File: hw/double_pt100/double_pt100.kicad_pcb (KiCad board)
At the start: 2 copper layers, 88.9 x 45.7 mm, 30 parts, among them SW1 SW_Push, U1 WeMos_D1_mini, U2 OLED_091_module, U3 MAX31865_breakout, U4 MAX31865_breakout

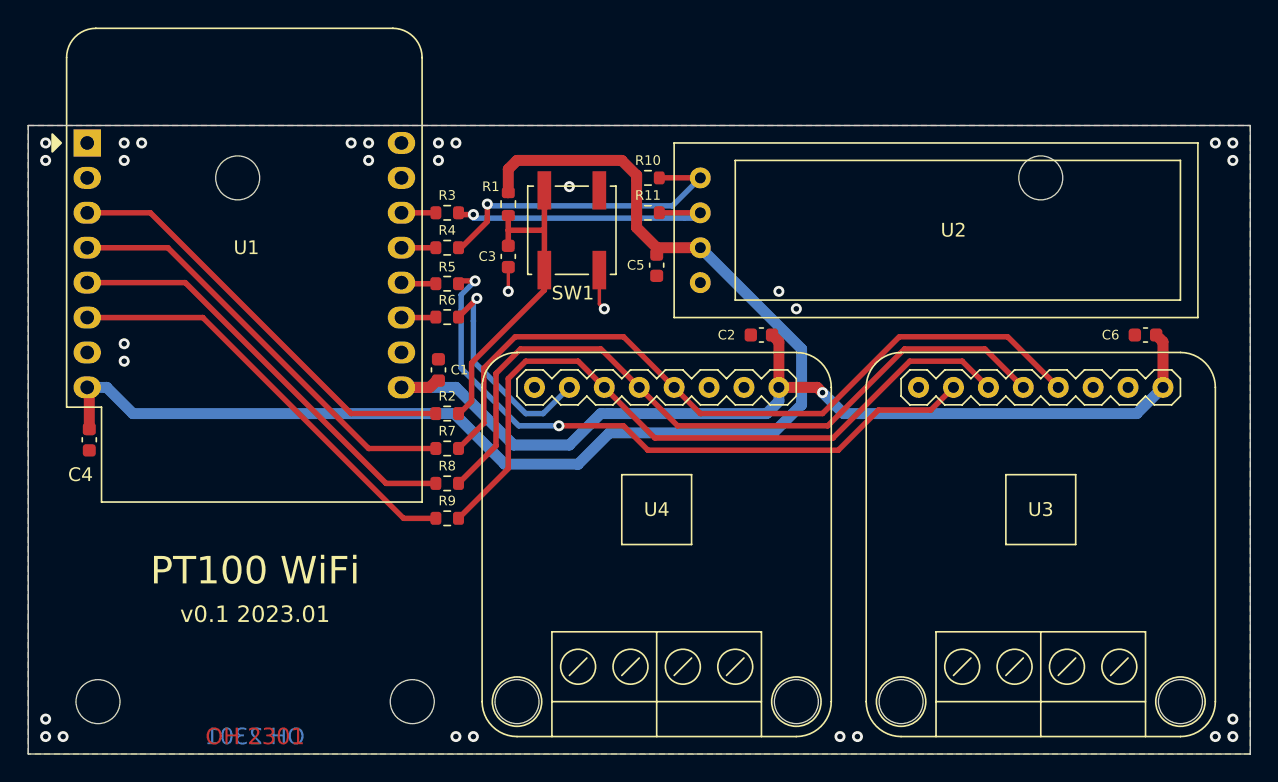
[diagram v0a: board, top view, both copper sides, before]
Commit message: hw version mini
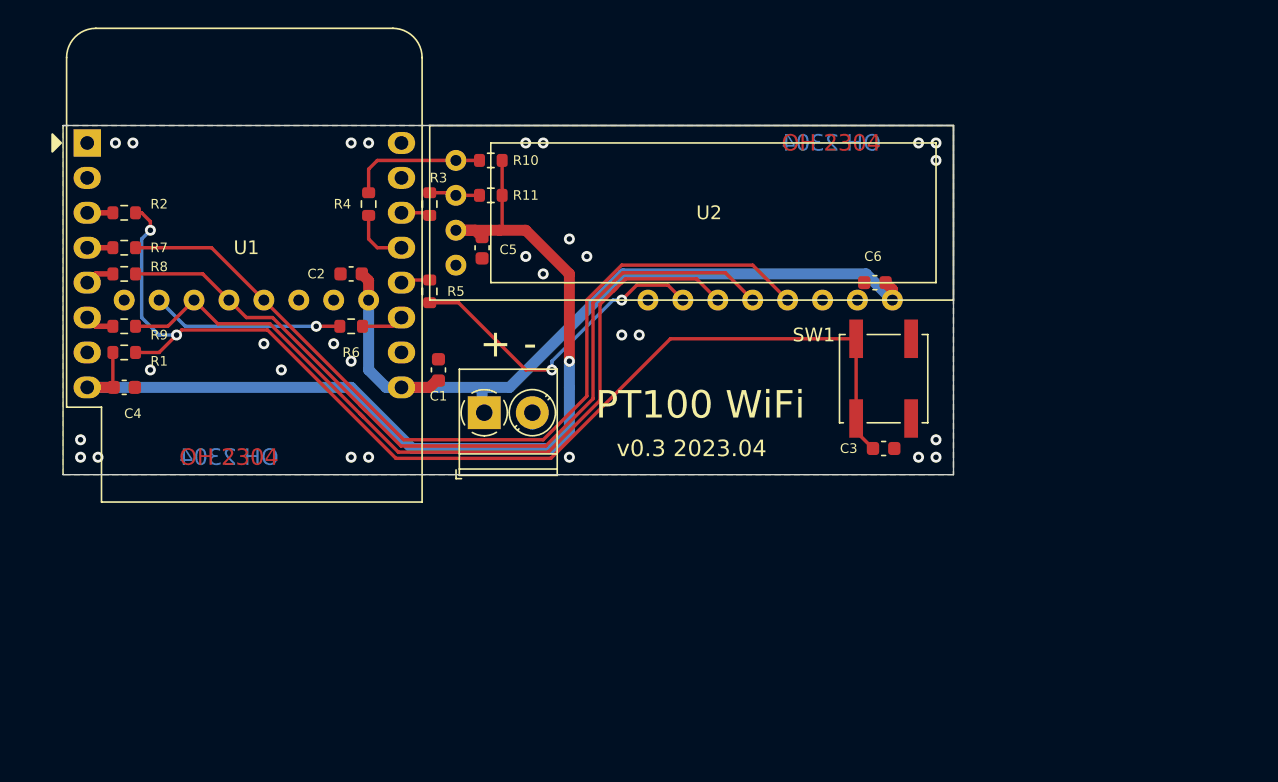
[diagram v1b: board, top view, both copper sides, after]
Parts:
- removed H1, H2, H3, H4, H5, H6, H7, H8: MountingHole, MountingHole:MountingHole_3.2mm_M3
- added J1: Screw_Terminal_01x02, TerminalBlock_Phoenix:TerminalBlock_Phoenix_PT-1,5-2-3.5-H_1x02_P3.50mm_Horizontal, F.Cu at (106.8, 125.0)
- moved C3 30.7 mm to (135.9, 127.6), turned to 0 degrees
- moved U4 30.5 mm to (88.3, 121.9)
- moved C2 30.2 mm to (97.2, 114.9)
- moved R1 30.0 mm to (80.6, 120.7), turned to 0 degrees
- moved R8 28.0 mm to (80.6, 114.9)
- moved R2 27.7 mm to (80.6, 110.5)
- moved R7 27.7 mm to (80.6, 113.0)
- moved R9 27.3 mm to (80.6, 118.7)
- moved SW1 25.1 mm to (135.9, 122.6)
- moved U3 20.7 mm to (126.4, 121.9)
- moved C6 20.1 mm to (135.3, 115.6)
- moved U2 17.8 mm to (104.8, 110.5)
- moved C5 12.8 mm to (106.7, 113.0)
- moved R10 11.5 mm to (107.3, 106.7), turned to 180 degrees
- moved R11 11.5 mm to (107.3, 109.2), turned to 180 degrees
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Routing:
- net SW: track 23.7 -> 80.7 mm, vias 0 -> 2
- net Net-(R7-Pad1): track 31.4 -> 1.86 mm
- net Net-(R2-Pad1): track 31.4 -> 1.86 mm
- net Net-(R8-Pad1): track 31.4 -> 2.13 mm
- net Net-(R9-Pad1): track 31.4 -> 2.13 mm
- net +3V3: track 95.0 -> 70.4 mm, vias 0 -> 1
- net CS1: track 48.2 -> 23.8 mm
- net SCL: track 21.0 -> 3.70 mm, vias 1 -> 0
- net +5V: track 72.0 -> 56.3 mm, vias 1 -> 0
- net SDA: track 23.5 -> 10.0 mm, vias 1 -> 0
- net CLK: track 55.5 -> 63.6 mm
- net SDO: track 54.0 -> 60.8 mm
- net SDI: track 52.5 -> 58.4 mm
- net GND: track 4.73 -> 1.58 mm, vias 31 -> 29
- net CS2: track 15.9 -> 13.9 mm
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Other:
- board size 88.9 x 45.7 mm -> 64.8 x 25.4 mm
- board text added: "+ -"
- board text added: "OH 2304"
- board text added: "v0.3 2023.04"
- board text removed: "OH 2301"
- board text removed: "v0.1 2023.01"
